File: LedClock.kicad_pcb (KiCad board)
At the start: 2 copper layers, 100 x 100 mm, 148 parts, among them J1 USB_B_Micro, J2 STM32_Debug, Q1 NJL7502R, SW1 Rotary_Encoder, U1 PCA9635, U2 PCA9635, U3 PCA9635, U4 PCA9635, U5 NJM78L33SU3, U6 STM32F303K8Tx, X1 12MHz

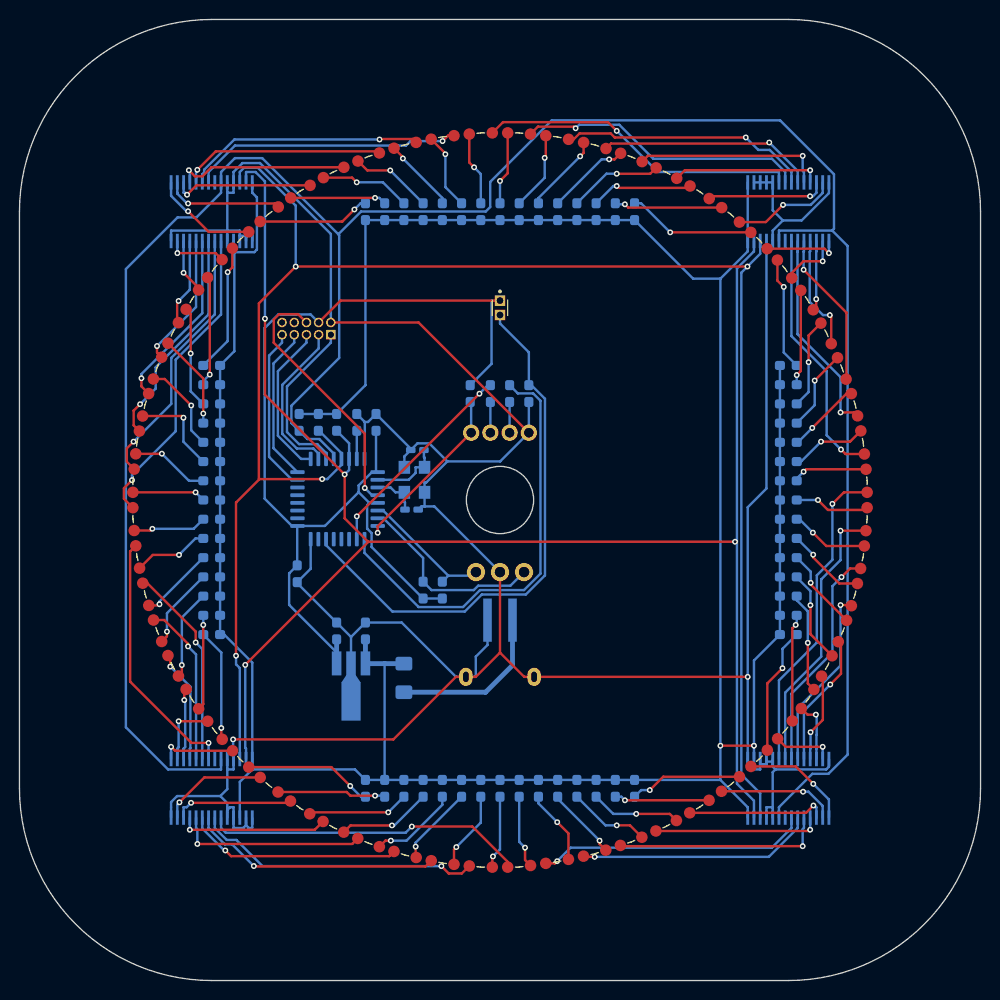
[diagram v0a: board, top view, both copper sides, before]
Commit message: 基板 V1.1
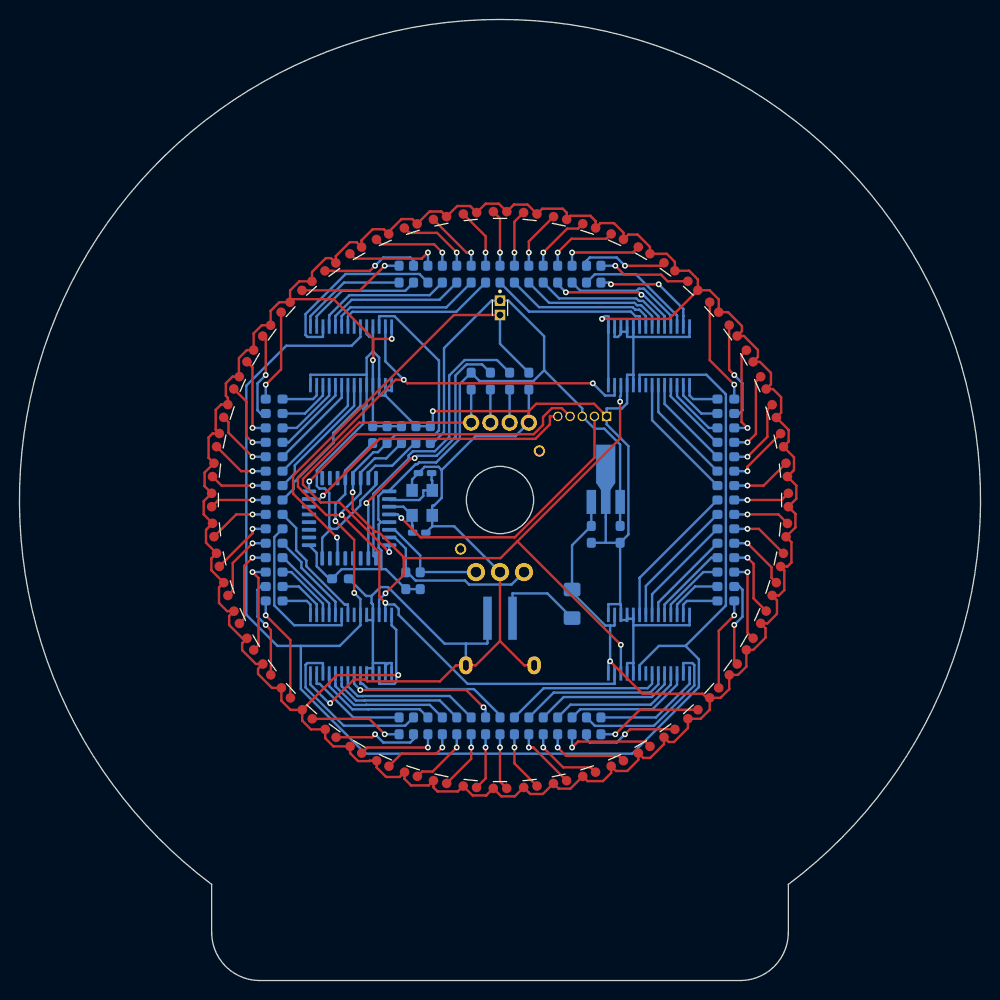
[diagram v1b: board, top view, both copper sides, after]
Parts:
- J2: footprint Connector_PinHeader_1.27mm:PinHeader_2x05_P1.27mm_Vertical -> LedClock:STM32_Debug_5pin
- moved U5 33.7 mm to (11.0, -1.78), turned to 90 degrees
- moved C2 31.2 mm to (12.5, 3.58), turned to 270 degrees
- moved J2 29.9 mm to (11.1, -8.70)
- moved C1 25.6 mm to (9.50, 3.58), turned to 270 degrees
- moved U1 20.9 mm to (15.5, -15.0)
- moved U2 20.9 mm to (15.5, 15.0)
- moved U3 20.9 mm to (-15.5, 15.0)
- moved U4 20.9 mm to (-15.5, -15.0)
- moved F1 19.1 mm to (7.50, 10.8)
- moved D57 8.25 mm to (-13.7, -26.8)
- moved D56 8.25 mm to (-16.4, -25.2)
- moved D54 8.25 mm to (-21.2, -21.2)
- moved D55 8.24 mm to (-18.9, -23.3)
- moved D58 8.24 mm to (-10.8, -28.0)
- moved D53 8.23 mm to (-23.4, -18.9)
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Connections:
- D1 pad 2: Net-(D1-Pad2) -> +5V
- D10 pad 2: Net-(D10-Pad2) -> +5V
- D11 pad 2: Net-(D11-Pad2) -> +5V
- D12 pad 2: Net-(D12-Pad2) -> +5V
- D13 pad 2: Net-(D13-Pad2) -> +5V
- D14 pad 2: Net-(D14-Pad2) -> +5V
- D15 pad 2: Net-(D15-Pad2) -> +5V
- D16 pad 2: Net-(D16-Pad2) -> +5V
- D17 pad 2: Net-(D17-Pad2) -> +5V
- D18 pad 2: Net-(D18-Pad2) -> +5V
- D19 pad 2: Net-(D19-Pad2) -> +5V
- D2 pad 2: Net-(D2-Pad2) -> +5V
- D20 pad 2: Net-(D20-Pad2) -> +5V
- D21 pad 2: Net-(D21-Pad2) -> +5V
- D22 pad 2: Net-(D22-Pad2) -> +5V
- D23 pad 2: Net-(D23-Pad2) -> +5V
- D24 pad 2: Net-(D24-Pad2) -> +5V
- D25 pad 2: Net-(D25-Pad2) -> +5V
- D26 pad 2: Net-(D26-Pad2) -> +5V
- D27 pad 2: Net-(D27-Pad2) -> +5V
- D28 pad 2: Net-(D28-Pad2) -> +5V
- D29 pad 2: Net-(D29-Pad2) -> +5V
- D3 pad 2: Net-(D3-Pad2) -> +5V
- D30 pad 2: Net-(D30-Pad2) -> +5V
- D31 pad 2: Net-(D31-Pad2) -> +5V
- D32 pad 2: Net-(D32-Pad2) -> +5V
- D33 pad 2: Net-(D33-Pad2) -> +5V
- D34 pad 2: Net-(D34-Pad2) -> +5V
- D35 pad 2: Net-(D35-Pad2) -> +5V
- D36 pad 2: Net-(D36-Pad2) -> +5V
- D37 pad 2: Net-(D37-Pad2) -> +5V
- D38 pad 2: Net-(D38-Pad2) -> +5V
- D39 pad 2: Net-(D39-Pad2) -> +5V
- D4 pad 2: Net-(D4-Pad2) -> +5V
- D40 pad 2: Net-(D40-Pad2) -> +5V
- D41 pad 2: Net-(D41-Pad2) -> +5V
- D42 pad 2: Net-(D42-Pad2) -> +5V
- D43 pad 2: Net-(D43-Pad2) -> +5V
- D44 pad 2: Net-(D44-Pad2) -> +5V
- D45 pad 2: Net-(D45-Pad2) -> +5V
- D46 pad 2: Net-(D46-Pad2) -> +5V
- D47 pad 2: Net-(D47-Pad2) -> +5V
- D48 pad 2: Net-(D48-Pad2) -> +5V
- D49 pad 2: Net-(D49-Pad2) -> +5V
- D5 pad 2: Net-(D5-Pad2) -> +5V
- D50 pad 2: Net-(D50-Pad2) -> +5V
- D51 pad 2: Net-(D51-Pad2) -> +5V
- D52 pad 2: Net-(D52-Pad2) -> +5V
- D53 pad 2: Net-(D53-Pad2) -> +5V
- D54 pad 2: Net-(D54-Pad2) -> +5V
- D55 pad 2: Net-(D55-Pad2) -> +5V
- D56 pad 2: Net-(D56-Pad2) -> +5V
- D57 pad 2: Net-(D57-Pad2) -> +5V
- D58 pad 2: Net-(D58-Pad2) -> +5V
- D59 pad 2: Net-(D59-Pad2) -> +5V
- D6 pad 2: Net-(D6-Pad2) -> +5V
- D60 pad 2: Net-(D60-Pad2) -> +5V
- D7 pad 2: Net-(D7-Pad2) -> +5V
- D8 pad 2: Net-(D8-Pad2) -> +5V
- D9 pad 2: Net-(D9-Pad2) -> +5V
- J2 pad 1: TRST -> GND
- J2 pad 2: GND -> NRST
- J2 pad 3: SWO -> +3V3
- J2 pad 4: +3V3 -> SWCLK
- J2 pad 5: TDI -> SWDIO
- R1 pad 1: +5V -> Net-(D1-Pad1)
- R1 pad 2: Net-(D1-Pad2) -> Net-(R1-Pad2)
- R10 pad 1: +5V -> Net-(D10-Pad1)
- R10 pad 2: Net-(D10-Pad2) -> Net-(R10-Pad2)
- R11 pad 1: +5V -> Net-(D11-Pad1)
- R11 pad 2: Net-(D11-Pad2) -> Net-(R11-Pad2)
- R12 pad 1: +5V -> Net-(D12-Pad1)
- R12 pad 2: Net-(D12-Pad2) -> Net-(R12-Pad2)
- R13 pad 1: +5V -> Net-(D13-Pad1)
- R13 pad 2: Net-(D13-Pad2) -> Net-(R13-Pad2)
- R14 pad 1: +5V -> Net-(D14-Pad1)
- R14 pad 2: Net-(D14-Pad2) -> Net-(R14-Pad2)
- R15 pad 1: +5V -> Net-(D15-Pad1)
- R15 pad 2: Net-(D15-Pad2) -> Net-(R15-Pad2)
- R16 pad 1: +5V -> Net-(D16-Pad1)
- R16 pad 2: Net-(D16-Pad2) -> Net-(R16-Pad2)
- R17 pad 1: +5V -> Net-(D17-Pad1)
- R17 pad 2: Net-(D17-Pad2) -> Net-(R17-Pad2)
- R18 pad 1: +5V -> Net-(D18-Pad1)
- R18 pad 2: Net-(D18-Pad2) -> Net-(R18-Pad2)
- R19 pad 1: +5V -> Net-(D19-Pad1)
- R19 pad 2: Net-(D19-Pad2) -> Net-(R19-Pad2)
- R2 pad 1: +5V -> Net-(D2-Pad1)
- R2 pad 2: Net-(D2-Pad2) -> Net-(R2-Pad2)
- R20 pad 1: +5V -> Net-(D20-Pad1)
- R20 pad 2: Net-(D20-Pad2) -> Net-(R20-Pad2)
- R21 pad 1: +5V -> Net-(D21-Pad1)
- R21 pad 2: Net-(D21-Pad2) -> Net-(R21-Pad2)
- R22 pad 1: +5V -> Net-(D22-Pad1)
- R22 pad 2: Net-(D22-Pad2) -> Net-(R22-Pad2)
- R23 pad 1: +5V -> Net-(D23-Pad1)
- R23 pad 2: Net-(D23-Pad2) -> Net-(R23-Pad2)
- R24 pad 1: +5V -> Net-(D24-Pad1)
- R24 pad 2: Net-(D24-Pad2) -> Net-(R24-Pad2)
- R25 pad 1: +5V -> Net-(D25-Pad1)
- R25 pad 2: Net-(D25-Pad2) -> Net-(R25-Pad2)
- R26 pad 1: +5V -> Net-(D26-Pad1)
- R26 pad 2: Net-(D26-Pad2) -> Net-(R26-Pad2)
- R27 pad 1: +5V -> Net-(D27-Pad1)
- R27 pad 2: Net-(D27-Pad2) -> Net-(R27-Pad2)
- R28 pad 1: +5V -> Net-(D28-Pad1)
- R28 pad 2: Net-(D28-Pad2) -> Net-(R28-Pad2)
- R29 pad 1: +5V -> Net-(D29-Pad1)
- R29 pad 2: Net-(D29-Pad2) -> Net-(R29-Pad2)
- R3 pad 1: +5V -> Net-(D3-Pad1)
- R3 pad 2: Net-(D3-Pad2) -> Net-(R3-Pad2)
- R30 pad 1: +5V -> Net-(D30-Pad1)
- R30 pad 2: Net-(D30-Pad2) -> Net-(R30-Pad2)
- R31 pad 1: +5V -> Net-(D31-Pad1)
- R31 pad 2: Net-(D31-Pad2) -> Net-(R31-Pad2)
- R32 pad 1: +5V -> Net-(D32-Pad1)
- R32 pad 2: Net-(D32-Pad2) -> Net-(R32-Pad2)
- R33 pad 1: +5V -> Net-(D33-Pad1)
- R33 pad 2: Net-(D33-Pad2) -> Net-(R33-Pad2)
- R34 pad 1: +5V -> Net-(D34-Pad1)
- R34 pad 2: Net-(D34-Pad2) -> Net-(R34-Pad2)
- R35 pad 1: +5V -> Net-(D35-Pad1)
- R35 pad 2: Net-(D35-Pad2) -> Net-(R35-Pad2)
- R36 pad 1: +5V -> Net-(D36-Pad1)
- R36 pad 2: Net-(D36-Pad2) -> Net-(R36-Pad2)
- R37 pad 1: +5V -> Net-(D37-Pad1)
- R37 pad 2: Net-(D37-Pad2) -> Net-(R37-Pad2)
- R38 pad 1: +5V -> Net-(D38-Pad1)
- R38 pad 2: Net-(D38-Pad2) -> Net-(R38-Pad2)
- R39 pad 1: +5V -> Net-(D39-Pad1)
- R39 pad 2: Net-(D39-Pad2) -> Net-(R39-Pad2)
- R4 pad 1: +5V -> Net-(D4-Pad1)
- R4 pad 2: Net-(D4-Pad2) -> Net-(R4-Pad2)
- R40 pad 1: +5V -> Net-(D40-Pad1)
- R40 pad 2: Net-(D40-Pad2) -> Net-(R40-Pad2)
- R41 pad 1: +5V -> Net-(D41-Pad1)
- R41 pad 2: Net-(D41-Pad2) -> Net-(R41-Pad2)
- R42 pad 1: +5V -> Net-(D42-Pad1)
- R42 pad 2: Net-(D42-Pad2) -> Net-(R42-Pad2)
- R43 pad 1: +5V -> Net-(D43-Pad1)
- R43 pad 2: Net-(D43-Pad2) -> Net-(R43-Pad2)
- R44 pad 1: +5V -> Net-(D44-Pad1)
- R44 pad 2: Net-(D44-Pad2) -> Net-(R44-Pad2)
- R45 pad 1: +5V -> Net-(D45-Pad1)
- R45 pad 2: Net-(D45-Pad2) -> Net-(R45-Pad2)
- R46 pad 1: +5V -> Net-(D46-Pad1)
- R46 pad 2: Net-(D46-Pad2) -> Net-(R46-Pad2)
- R47 pad 1: +5V -> Net-(D47-Pad1)
- R47 pad 2: Net-(D47-Pad2) -> Net-(R47-Pad2)
- R48 pad 1: +5V -> Net-(D48-Pad1)
- R48 pad 2: Net-(D48-Pad2) -> Net-(R48-Pad2)
- R49 pad 1: +5V -> Net-(D49-Pad1)
- R49 pad 2: Net-(D49-Pad2) -> Net-(R49-Pad2)
- R5 pad 1: +5V -> Net-(D5-Pad1)
- R5 pad 2: Net-(D5-Pad2) -> Net-(R5-Pad2)
- R50 pad 1: +5V -> Net-(D50-Pad1)
- R50 pad 2: Net-(D50-Pad2) -> Net-(R50-Pad2)
- R51 pad 1: +5V -> Net-(D51-Pad1)
- R51 pad 2: Net-(D51-Pad2) -> Net-(R51-Pad2)
- R52 pad 1: +5V -> Net-(D52-Pad1)
- R52 pad 2: Net-(D52-Pad2) -> Net-(R52-Pad2)
- R53 pad 1: +5V -> Net-(D53-Pad1)
- R53 pad 2: Net-(D53-Pad2) -> Net-(R53-Pad2)
- R54 pad 1: +5V -> Net-(D54-Pad1)
- R54 pad 2: Net-(D54-Pad2) -> Net-(R54-Pad2)
- R55 pad 1: +5V -> Net-(D55-Pad1)
- R55 pad 2: Net-(D55-Pad2) -> Net-(R55-Pad2)
- R56 pad 1: +5V -> Net-(D56-Pad1)
- R56 pad 2: Net-(D56-Pad2) -> Net-(R56-Pad2)
- R57 pad 1: +5V -> Net-(D57-Pad1)
- R57 pad 2: Net-(D57-Pad2) -> Net-(R57-Pad2)
- R58 pad 1: +5V -> Net-(D58-Pad1)
- R58 pad 2: Net-(D58-Pad2) -> Net-(R58-Pad2)
- R59 pad 1: +5V -> Net-(D59-Pad1)
- R59 pad 2: Net-(D59-Pad2) -> Net-(R59-Pad2)
- R6 pad 1: +5V -> Net-(D6-Pad1)
- R6 pad 2: Net-(D6-Pad2) -> Net-(R6-Pad2)
- R60 pad 1: +5V -> Net-(D60-Pad1)
- R60 pad 2: Net-(D60-Pad2) -> Net-(R60-Pad2)
- R7 pad 1: +5V -> Net-(D7-Pad1)
- R7 pad 2: Net-(D7-Pad2) -> Net-(R7-Pad2)
- R8 pad 1: +5V -> Net-(D8-Pad1)
- R8 pad 2: Net-(D8-Pad2) -> Net-(R8-Pad2)
- R9 pad 1: +5V -> Net-(D9-Pad1)
- R9 pad 2: Net-(D9-Pad2) -> Net-(R9-Pad2)
- U1 pad 10: Net-(D5-Pad1) -> Net-(R5-Pad2)
- U1 pad 11: Net-(D6-Pad1) -> Net-(R6-Pad2)
- U1 pad 12: Net-(D7-Pad1) -> Net-(R7-Pad2)
- U1 pad 13: Net-(D8-Pad1) -> Net-(R8-Pad2)
- U1 pad 15: Net-(D9-Pad1) -> Net-(R9-Pad2)
- U1 pad 16: Net-(D10-Pad1) -> Net-(R10-Pad2)
- U1 pad 17: Net-(D11-Pad1) -> Net-(R11-Pad2)
- U1 pad 18: Net-(D12-Pad1) -> Net-(R12-Pad2)
- U1 pad 19: Net-(D13-Pad1) -> Net-(R13-Pad2)
- U1 pad 20: Net-(D14-Pad1) -> Net-(R14-Pad2)
- U1 pad 21: Net-(D15-Pad1) -> Net-(R15-Pad2)
- U1 pad 6: Net-(D1-Pad1) -> Net-(R1-Pad2)
- U1 pad 7: Net-(D2-Pad1) -> Net-(R2-Pad2)
- U1 pad 8: Net-(D3-Pad1) -> Net-(R3-Pad2)
- U1 pad 9: Net-(D4-Pad1) -> Net-(R4-Pad2)
- U2 pad 10: Net-(D20-Pad1) -> Net-(R20-Pad2)
- U2 pad 11: Net-(D21-Pad1) -> Net-(R21-Pad2)
- U2 pad 12: Net-(D22-Pad1) -> Net-(R22-Pad2)
- U2 pad 13: Net-(D23-Pad1) -> Net-(R23-Pad2)
- U2 pad 15: Net-(D24-Pad1) -> Net-(R24-Pad2)
- U2 pad 16: Net-(D25-Pad1) -> Net-(R25-Pad2)
- U2 pad 17: Net-(D26-Pad1) -> Net-(R26-Pad2)
- U2 pad 18: Net-(D27-Pad1) -> Net-(R27-Pad2)
- U2 pad 19: Net-(D28-Pad1) -> Net-(R28-Pad2)
- U2 pad 20: Net-(D29-Pad1) -> Net-(R29-Pad2)
- U2 pad 21: Net-(D30-Pad1) -> Net-(R30-Pad2)
- U2 pad 6: Net-(D16-Pad1) -> Net-(R16-Pad2)
- U2 pad 7: Net-(D17-Pad1) -> Net-(R17-Pad2)
- U2 pad 8: Net-(D18-Pad1) -> Net-(R18-Pad2)
- U2 pad 9: Net-(D19-Pad1) -> Net-(R19-Pad2)
- U3 pad 10: Net-(D35-Pad1) -> Net-(R35-Pad2)
- U3 pad 11: Net-(D36-Pad1) -> Net-(R36-Pad2)
- U3 pad 12: Net-(D37-Pad1) -> Net-(R37-Pad2)
- U3 pad 13: Net-(D38-Pad1) -> Net-(R38-Pad2)
- U3 pad 15: Net-(D39-Pad1) -> Net-(R39-Pad2)
- U3 pad 16: Net-(D40-Pad1) -> Net-(R40-Pad2)
- U3 pad 17: Net-(D41-Pad1) -> Net-(R41-Pad2)
- U3 pad 18: Net-(D42-Pad1) -> Net-(R42-Pad2)
- U3 pad 19: Net-(D43-Pad1) -> Net-(R43-Pad2)
- U3 pad 20: Net-(D44-Pad1) -> Net-(R44-Pad2)
- U3 pad 21: Net-(D45-Pad1) -> Net-(R45-Pad2)
- U3 pad 6: Net-(D31-Pad1) -> Net-(R31-Pad2)
- U3 pad 7: Net-(D32-Pad1) -> Net-(R32-Pad2)
- U3 pad 8: Net-(D33-Pad1) -> Net-(R33-Pad2)
- U3 pad 9: Net-(D34-Pad1) -> Net-(R34-Pad2)
- U4 pad 10: Net-(D50-Pad1) -> Net-(R50-Pad2)
- U4 pad 11: Net-(D51-Pad1) -> Net-(R51-Pad2)
- U4 pad 12: Net-(D52-Pad1) -> Net-(R52-Pad2)
- U4 pad 13: Net-(D53-Pad1) -> Net-(R53-Pad2)
- U4 pad 15: Net-(D54-Pad1) -> Net-(R54-Pad2)
- U4 pad 16: Net-(D55-Pad1) -> Net-(R55-Pad2)
- U4 pad 17: Net-(D56-Pad1) -> Net-(R56-Pad2)
- U4 pad 18: Net-(D57-Pad1) -> Net-(R57-Pad2)
- U4 pad 19: Net-(D58-Pad1) -> Net-(R58-Pad2)
- U4 pad 20: Net-(D59-Pad1) -> Net-(R59-Pad2)
- U4 pad 21: Net-(D60-Pad1) -> Net-(R60-Pad2)
- U4 pad 6: Net-(D46-Pad1) -> Net-(R46-Pad2)
- U4 pad 7: Net-(D47-Pad1) -> Net-(R47-Pad2)
- U4 pad 8: Net-(D48-Pad1) -> Net-(R48-Pad2)
- U4 pad 9: Net-(D49-Pad1) -> Net-(R49-Pad2)
- U6 pad 24: SWCLC -> SWCLK
- U6 pad 25: TDI -> (no net)
- U6 pad 26: SWO -> (no net)
- U6 pad 27: TRST -> (no net)
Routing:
- net SCL: track 191.5 -> 97.0 mm
- net LED_OE: track 258.5 -> 176.3 mm, vias 0 -> 2
- net GND: track 343.9 -> 266.6 mm
- net SDA: track 178.5 -> 103.7 mm
- net SWCLK: track 0.00 -> 32.2 mm, vias 0 -> 1
- net Net-(D1-Pad1): track 33.5 -> 5.91 mm
- net Net-(D31-Pad1): track 33.5 -> 5.91 mm
- net Net-(D16-Pad1): track 33.0 -> 5.91 mm
- net Net-(D46-Pad1): track 32.3 -> 5.91 mm
- net Net-(D2-Pad1): track 30.2 -> 5.93 mm
- net Net-(D32-Pad1): track 29.8 -> 5.92 mm
- net +5V: track 319.0 -> 342.3 mm, vias 2 -> 5
- net Net-(D17-Pad1): track 28.8 -> 5.92 mm
- net Net-(D47-Pad1): track 27.8 -> 5.92 mm
- net Net-(D60-Pad1): track 28.2 -> 6.34 mm
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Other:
- outline, holes or cut-outs redrawn
- board text added: "LED Clock V1.1"
- board text removed: "LED Clock V1.0"
